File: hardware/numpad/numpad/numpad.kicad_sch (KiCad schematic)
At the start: 5 parts, among them J1 Conn_01x04, J2 Conn_01x04, J3 Conn_01x04, J4 Conn_01x04, U1 STM32F446RET6

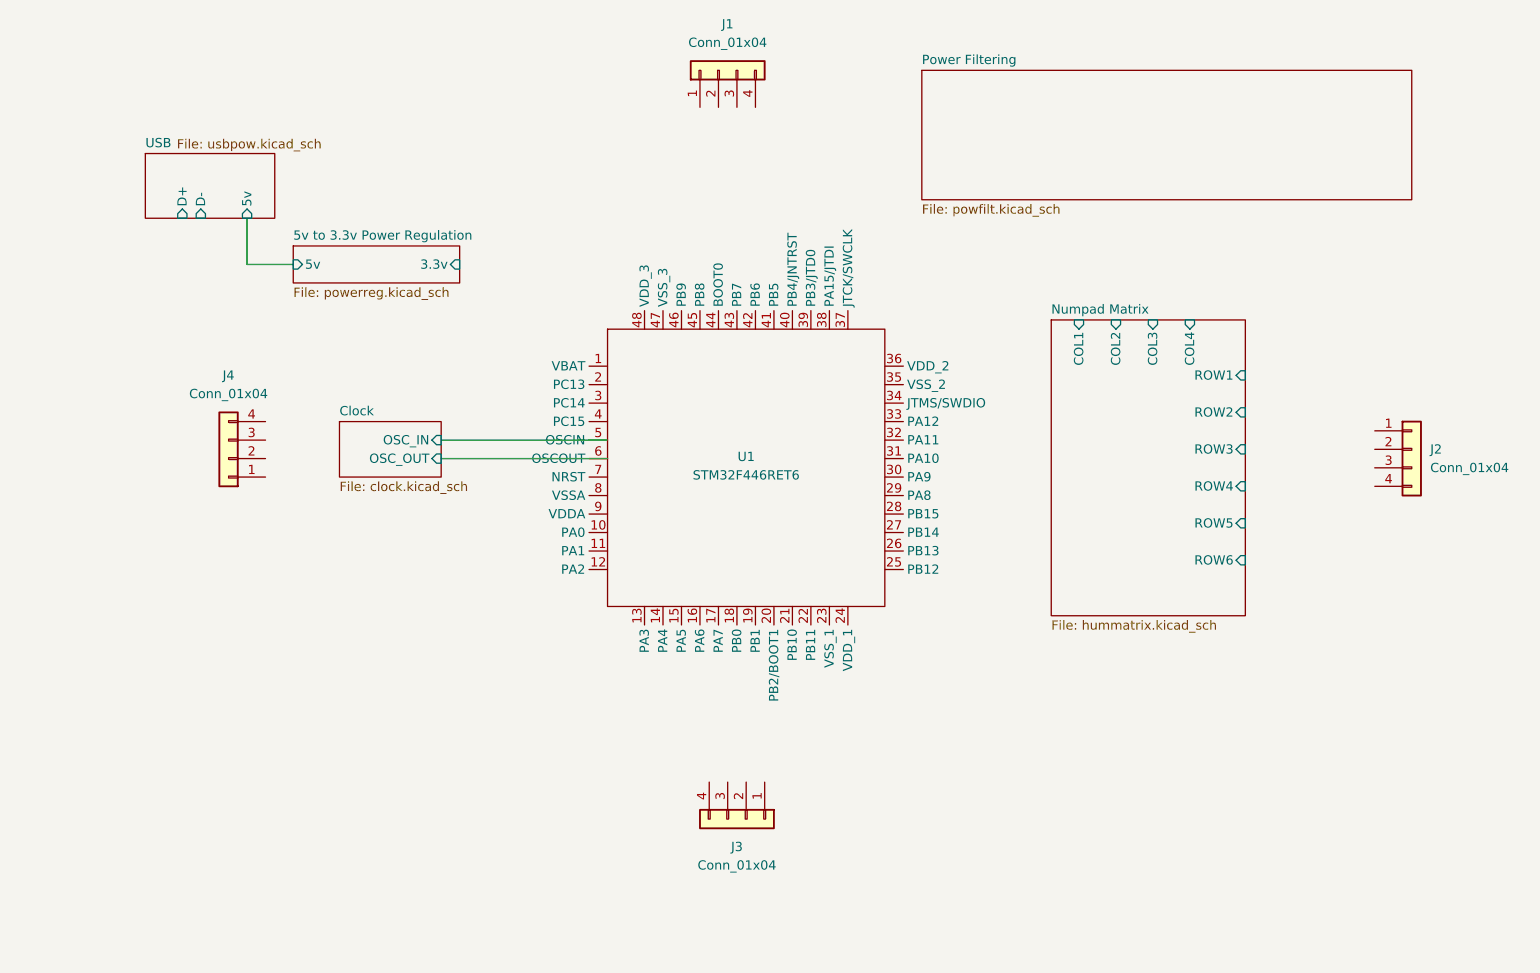
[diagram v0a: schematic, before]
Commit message: connectors for other modules
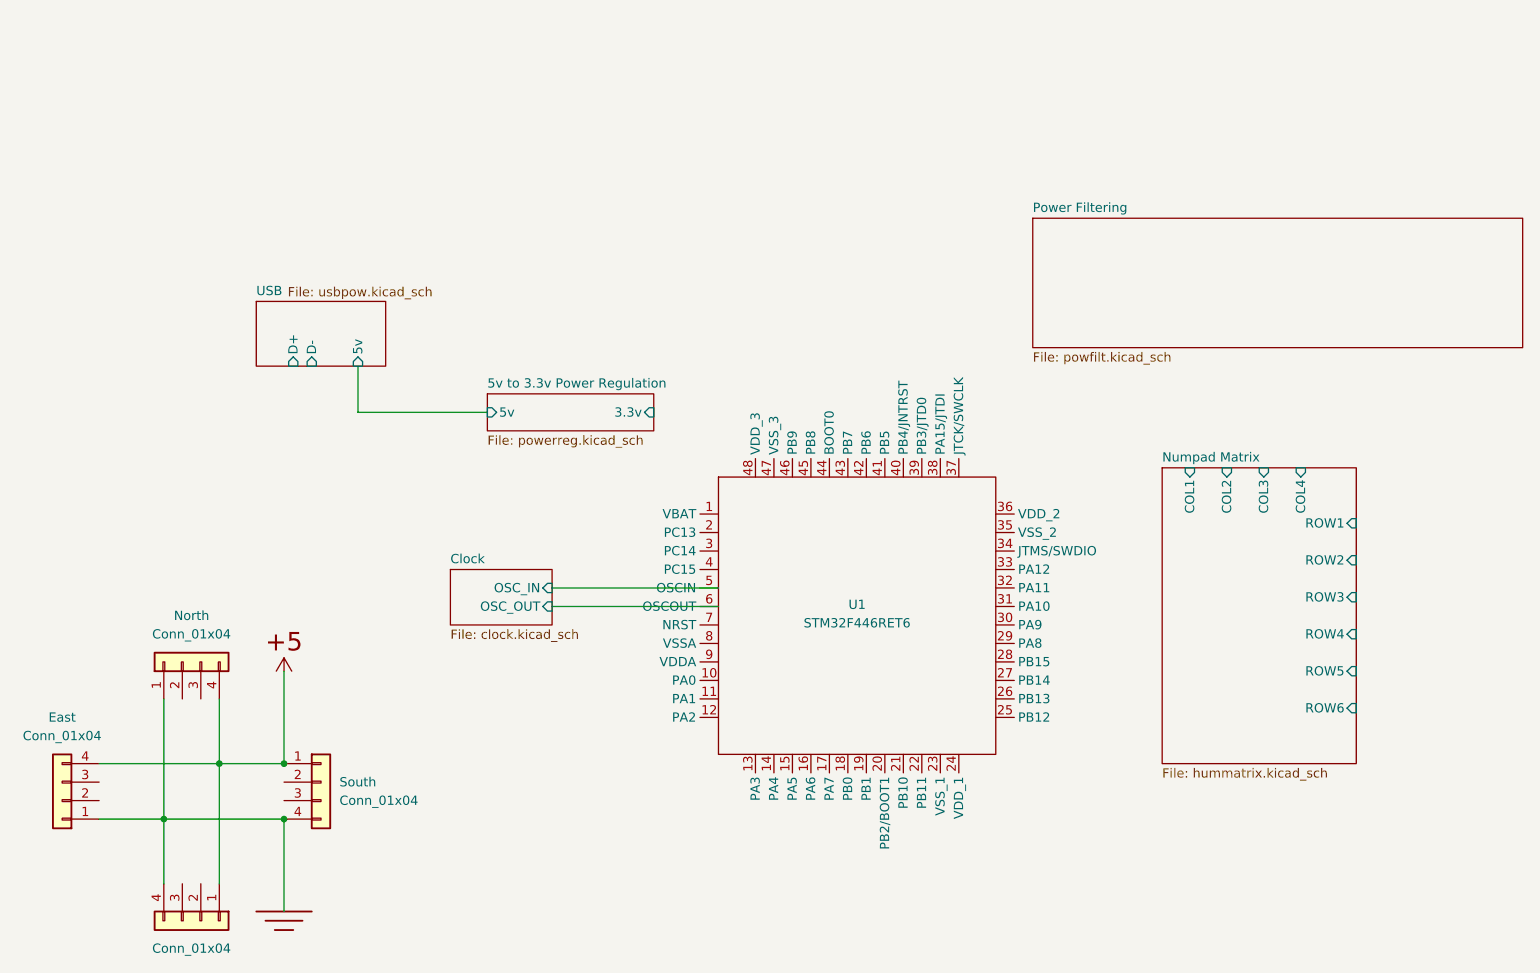
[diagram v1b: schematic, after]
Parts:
- renumbered J4 to East, J1 to North, J3 to South, J2 to West
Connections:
- net P,+5: now reaches South.1 (Pin_1)
- net P,+5: now also East.4 (Pin_4), North.4 (Pin_4), West.1 (Pin_1)
- net P,E: now reaches South.4 (Pin_4)
- net P,E: now also East.1 (Pin_1), North.1 (Pin_1), West.4 (Pin_4)
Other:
- moved on the sheet: East, North, South, U1
